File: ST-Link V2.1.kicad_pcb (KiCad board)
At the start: 2 copper layers, 31.8 x 20.9 mm, 46 parts, among them J1 USB_OTG, J2 Conn_01x06, J3 Conn_01x08, J4 Conn_01x08, Q1 MMBT3904, U1 USBLC6-2SC6, U2 stm32, U3 MIC5219-3.3, X1 8MHz

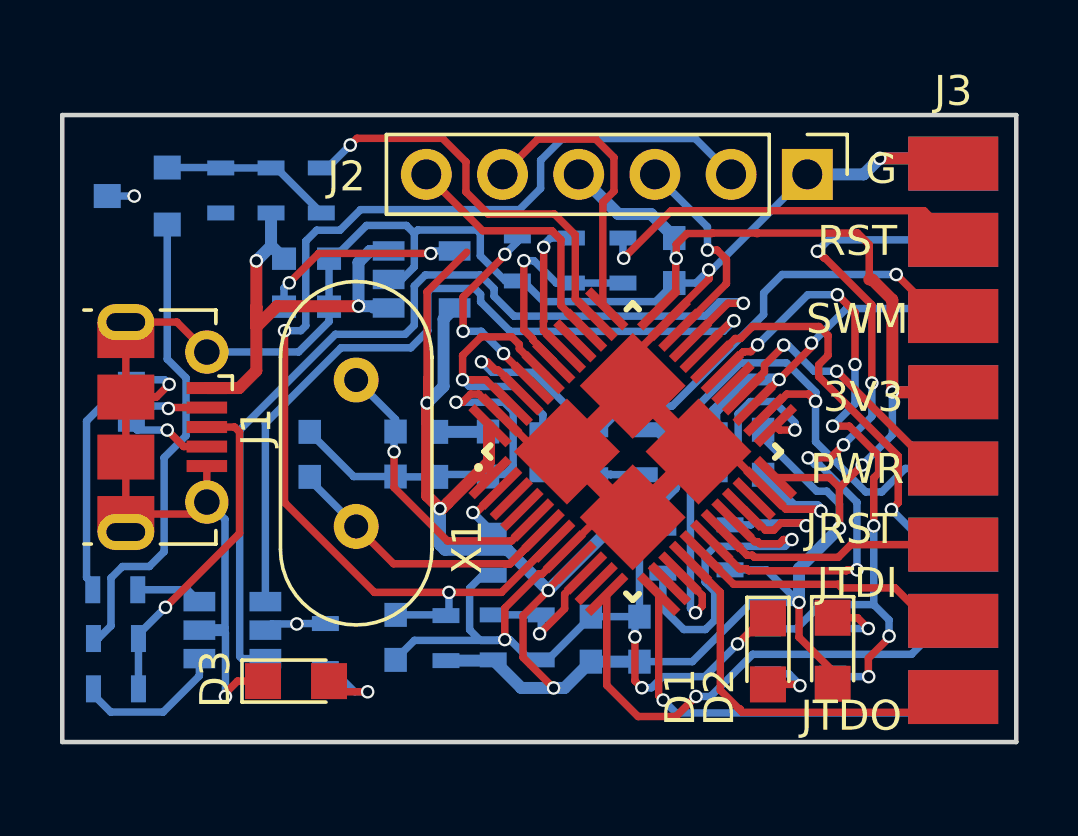
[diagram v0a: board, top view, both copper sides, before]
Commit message: added BOM,updated size and gerber file
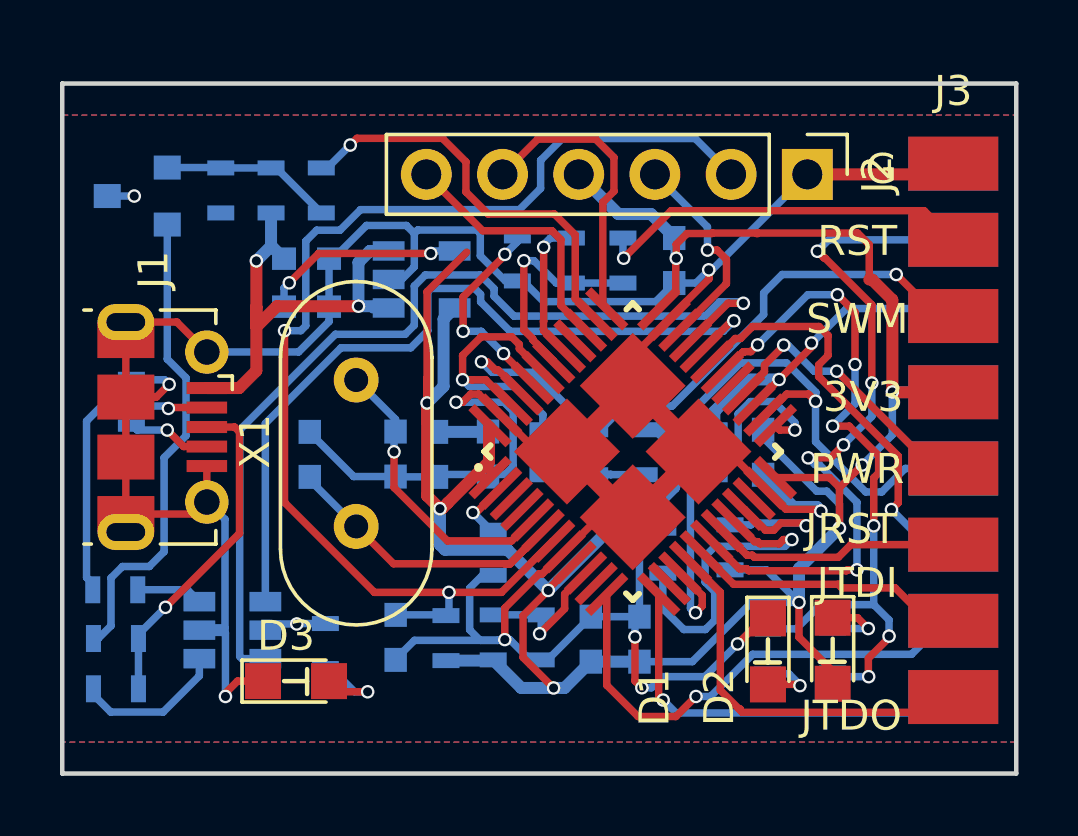
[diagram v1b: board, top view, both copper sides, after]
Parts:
- D1, D2, D3: footprint LEDs:LED_0805 -> MetalPad:LED_0805
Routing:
- net GND: track 138.8 -> 131.6 mm, vias 10 -> 9
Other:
- board size 31.8 x 20.9 mm -> 31.8 x 23 mm
